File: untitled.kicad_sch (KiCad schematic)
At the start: 14 parts, among them J5 Screw_Terminal_01x02, U3 LM2596S-ADJ, U4 TPS54560BDDA

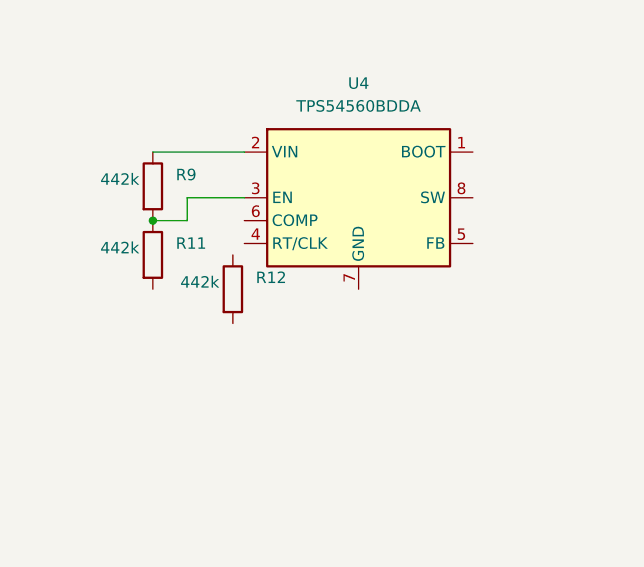
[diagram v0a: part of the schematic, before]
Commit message: Autosave
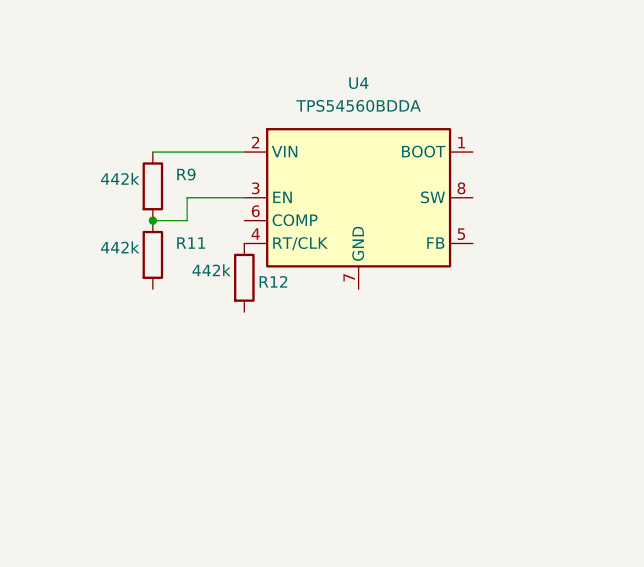
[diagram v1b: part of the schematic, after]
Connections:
- net at R12.1: now also U4.4 (RT/CLK)
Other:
- moved on the sheet: R12
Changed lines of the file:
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@@
 	(symbol
 		(lib_id "Device:R")
-		(at 78.74 53.34 0)
+		(at 80.01 52.07 0)
 		(unit 1)
 		(body_style 1)
@@
 		(dnp no)
 		(property "Reference" "R12"
-			(at 81.28 52.0699 0)
+			(at 81.534 52.578 0)
 			(show_name no)
 			(do_not_autoplace no)
@@
 		)
 		(property "Value" "442k"
-			(at 72.898 52.578 0)
+			(at 74.168 51.308 0)
 			(show_name no)
 			(do_not_autoplace no)
@@
 		)
 		(property "Footprint" ""
-			(at 76.962 53.34 90)
+			(at 78.232 52.07 90)
 			(hide yes)
 			(show_name no)
@@
 		)
 		(property "Datasheet" ""
-			(at 78.74 53.34 0)
+			(at 80.01 52.07 0)
 			(hide yes)
 			(show_name no)
@@
 		)
 		(property "Description" "Resistor"
-			(at 78.74 53.34 0)
+			(at 80.01 52.07 0)
 			(hide yes)
 			(show_name no)
